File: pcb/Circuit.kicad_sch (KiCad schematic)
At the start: 56 parts, among them J1 DTM13-12PA-R008, J2 TSW-101-07-T-D, J3 TSW-101-07-T-D, U1 MCP2561, U2 CDP68HC68S1, U3 LM2594HVM-5.0, U4 Teensy4.0

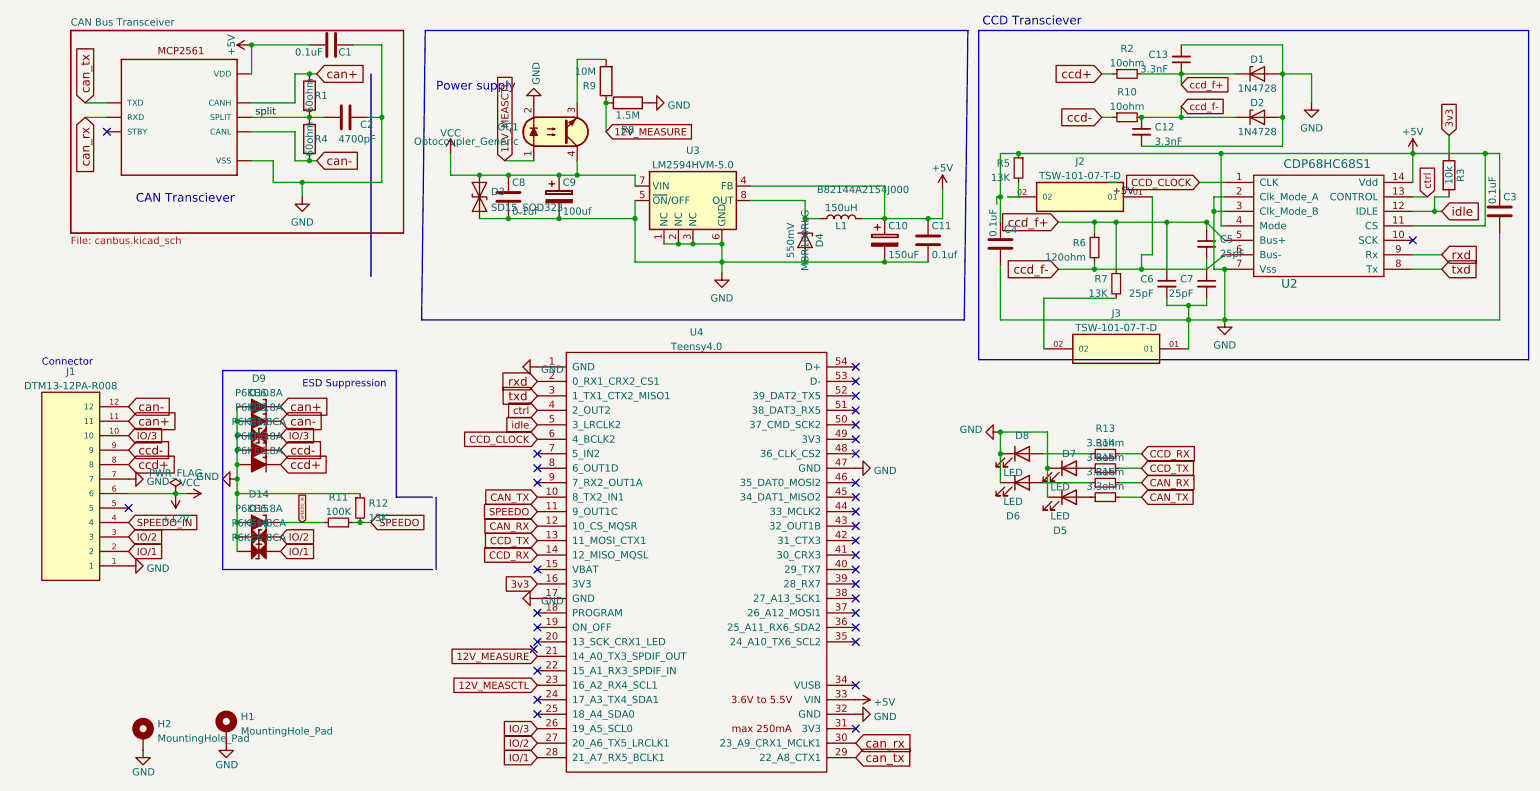
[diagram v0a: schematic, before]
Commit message: commit before changing can transceiver
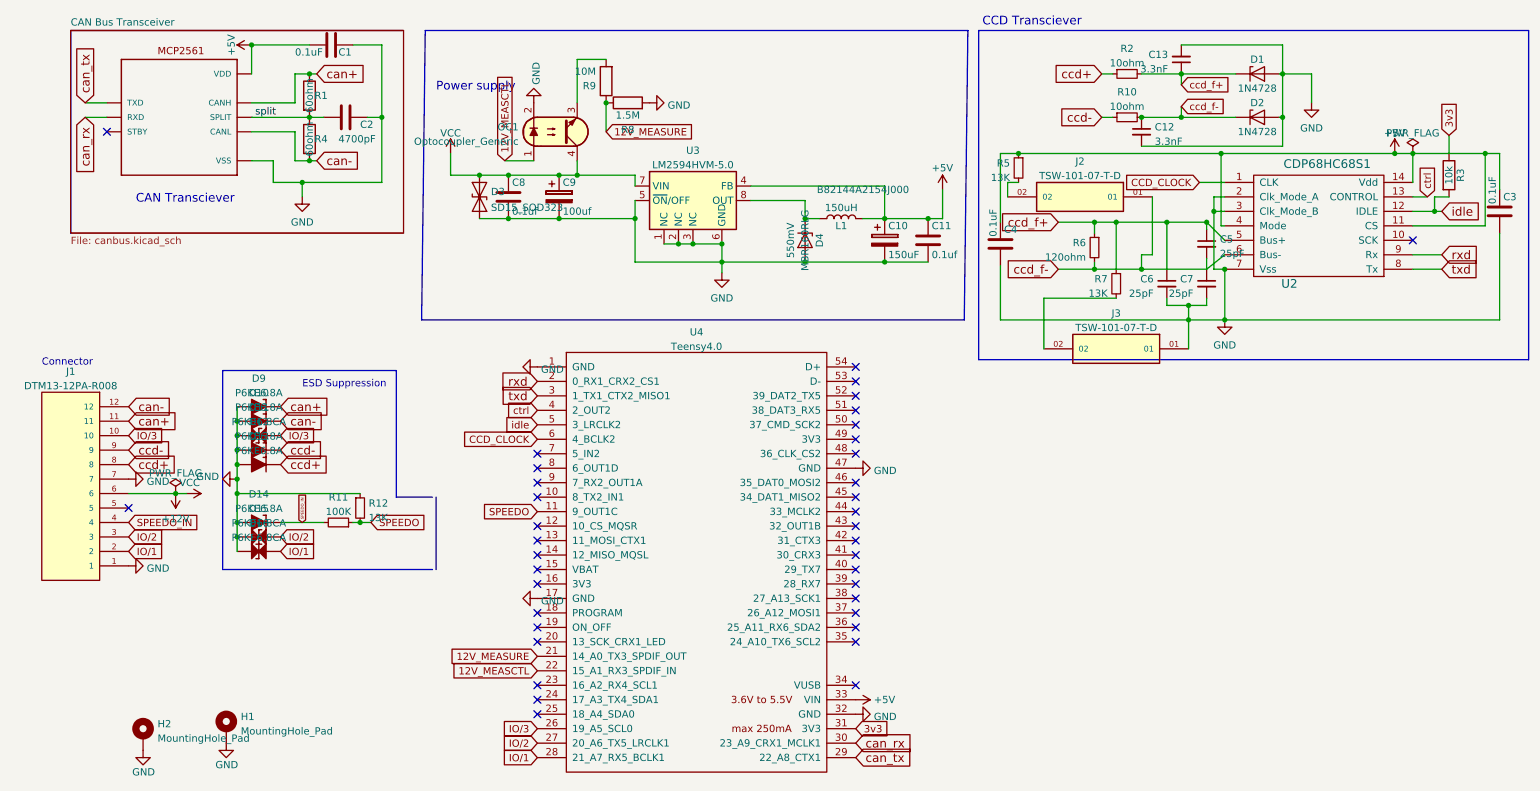
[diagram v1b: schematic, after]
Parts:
- removed D5, D6, D7, D8: LED, LED_SMD:LED_0805_2012Metric_Pad1.15x1.40mm_HandSolder, symbol Device:LED
- removed R13, R14, R15, R16: 3.3ohm, Resistor_SMD:R_0603_1608Metric_Pad0.98x0.95mm_HandSolder, symbol Device:R_Small
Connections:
- net 12V_MEASCTL: now also U4.22 (15_A1_RX3_SPDIF_IN); no longer U4.23 (16_A2_RX4_SCL1)
- net 3v3: now also U4.31 (3V3); no longer U4.16 (3V3)
- net CAN_RX: no longer names the net of U4.12 (10_CS_MQSR)
- net CAN_TX: no longer names the net of U4.10 (8_TX2_IN1)
- net CCD_RX: no longer names the net of U4.14 (12_MISO_MQSL)
- net CCD_TX: no longer names the net of U4.13 (11_MOSI_CTX1)
- no-connect marks 35 -> 38
